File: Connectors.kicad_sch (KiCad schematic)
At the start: 17 parts, among them J1 353630660, J2 353630660, U2 TJA1051T/3, U3 ICM-42688-P

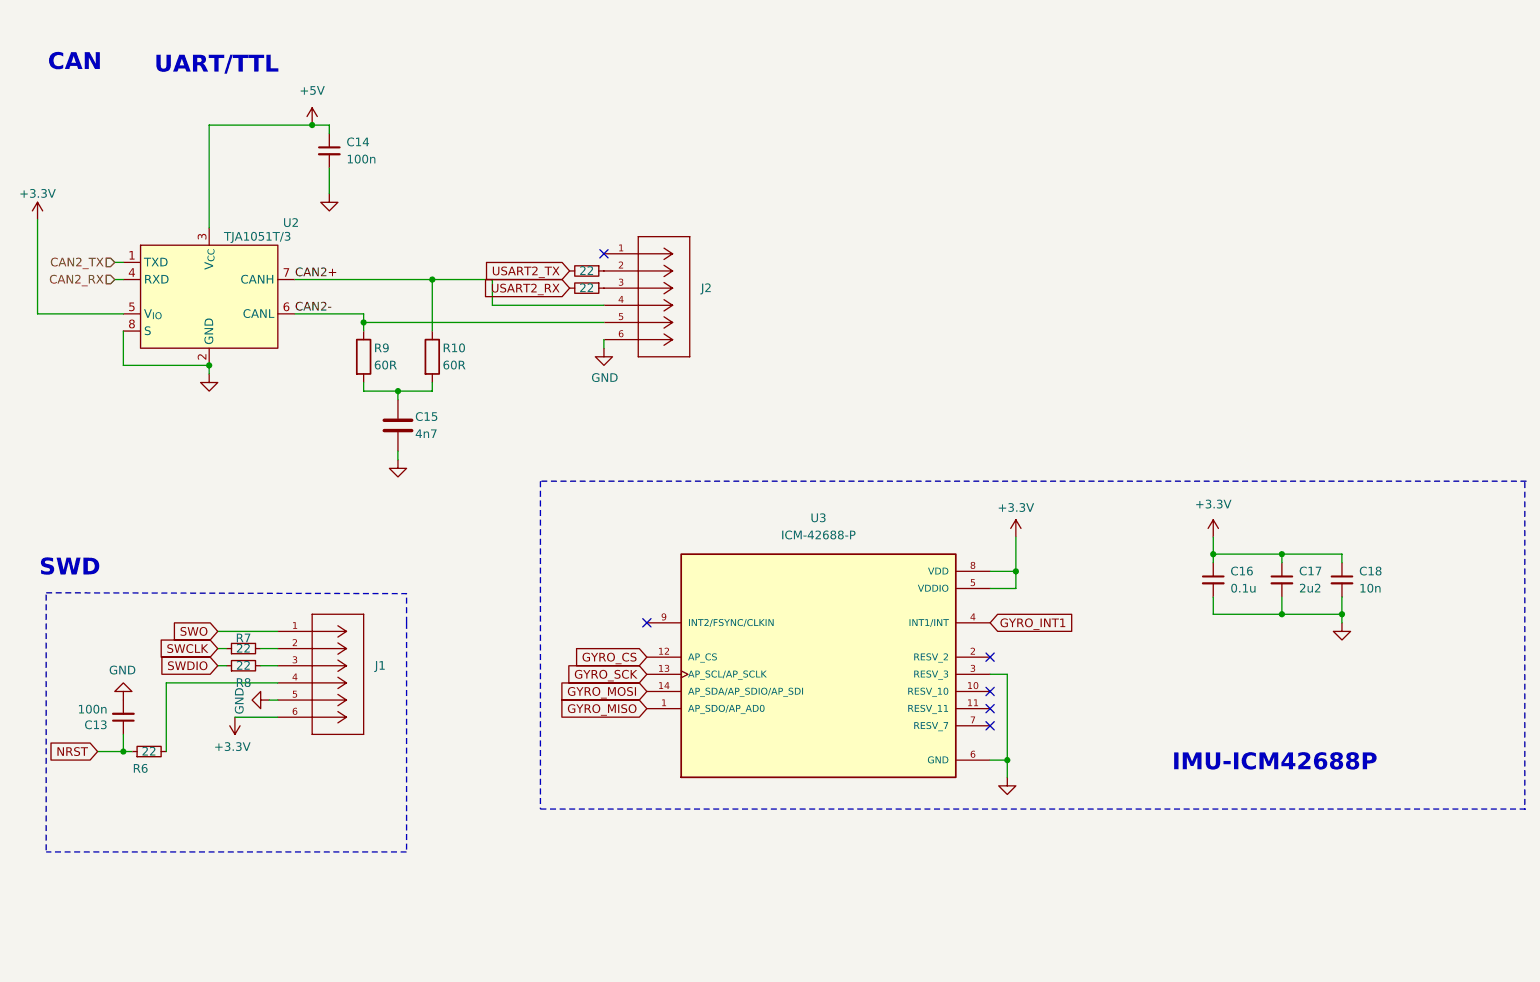
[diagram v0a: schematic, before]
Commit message: update
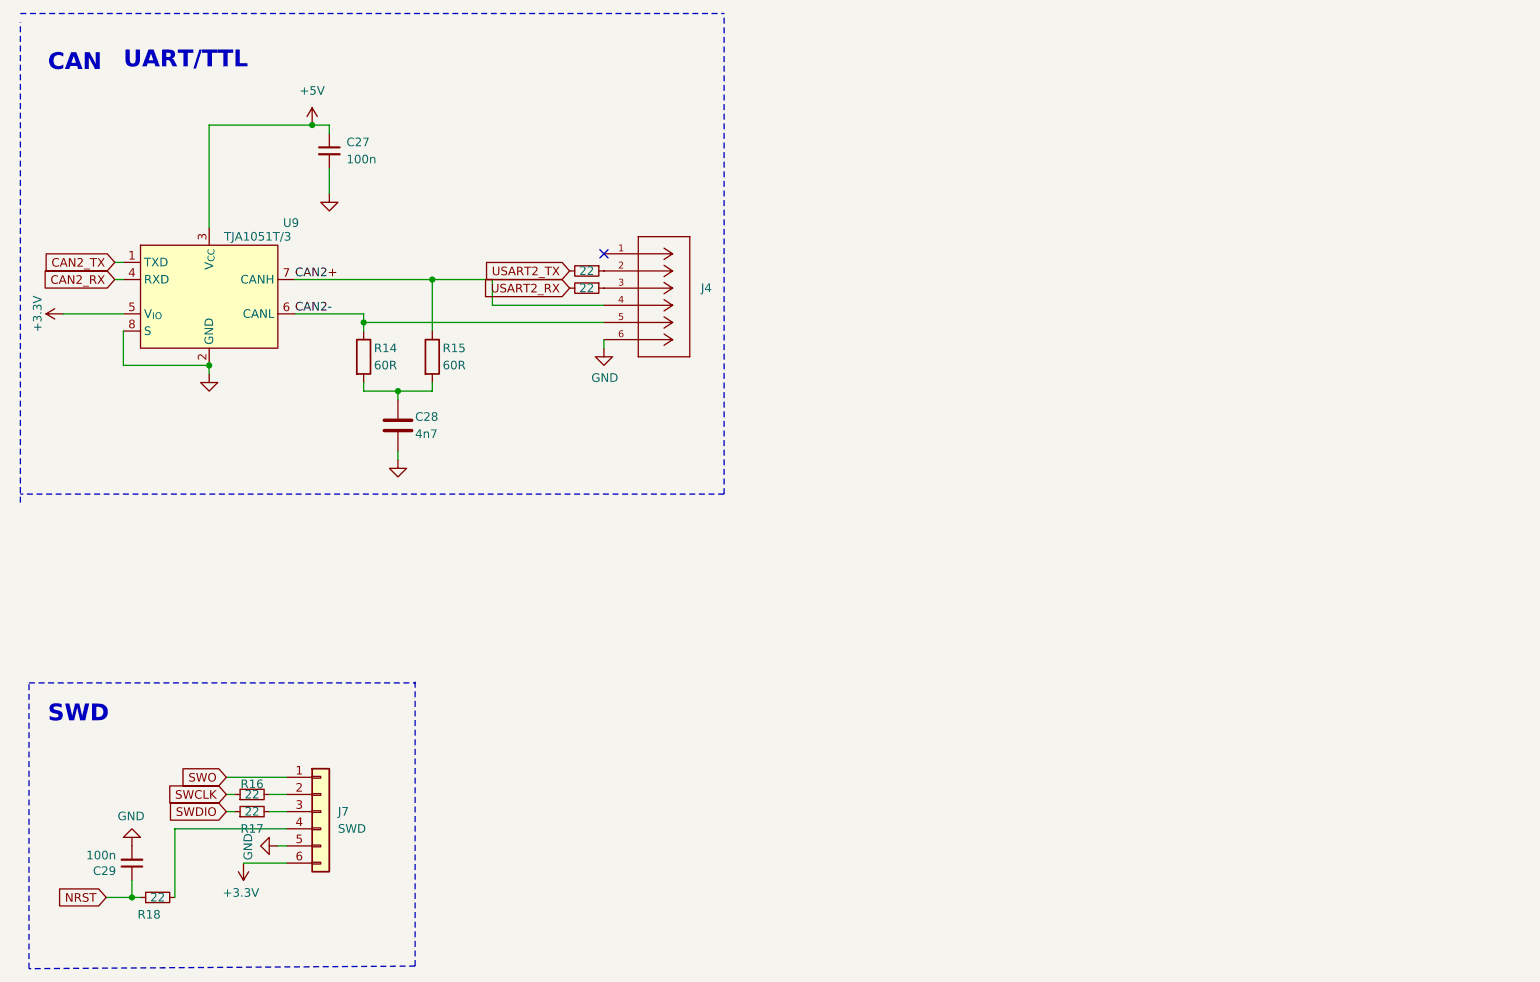
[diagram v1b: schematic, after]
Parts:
- removed C16: 0.1u, Capacitor_SMD:C_0402_1005Metric, symbol Device:C_Small
- removed C17: 2u2, Capacitor_SMD:C_0603_1608Metric, symbol Device:C_Small
- removed C18: 10n, Capacitor_SMD:C_0402_1005Metric, symbol Device:C_Small
- removed J1: 353630660, mylib:CON_353630660, symbol 353630660:353630660
- removed U3: ICM-42688-P, mylib:PQFN50P300X250X97-14N, symbol ICM-42688-P:ICM-42688-P
- added J7: SWD, Connector_PinHeader_2.54mm:PinHeader_1x06_P2.54mm_Vertical, symbol Connector_Generic:Conn_01x06
- renumbered C14 to C27, C15 to C28, C13 to C29, J2 to J4, R11 to R12, R12 to R13, R9 to R14, R10 to R15, R7 to R16, R8 to R17, R6 to R18, U2 to U9
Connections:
- net +3.3V: now also J7.6 (Pin_6)
- net GND: now also J7.5 (Pin_5)
- net SWO: now also J7.1 (Pin_1)
- net at R17.2: now also J7.3 (Pin_3)
- net at R16.2: now also J7.2 (Pin_2)
- net at R18.2: now also J7.4 (Pin_4)
- no-connect marks 6 -> 1
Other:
- note removed: "IMU-ICM42688P"
- moved on the sheet: C29, R16, R17, R18
